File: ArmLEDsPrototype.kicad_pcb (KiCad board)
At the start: 2 copper layers, 11 parts

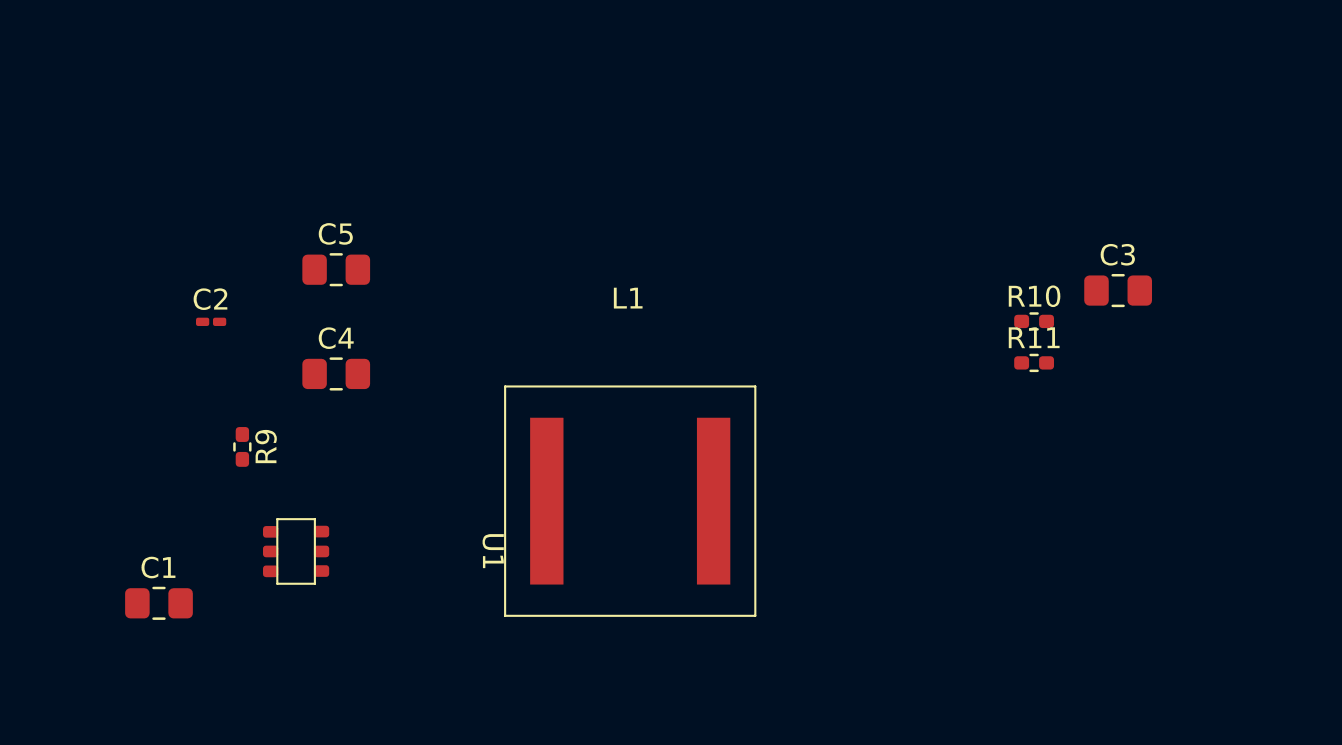
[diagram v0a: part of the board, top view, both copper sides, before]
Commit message: Making PCB
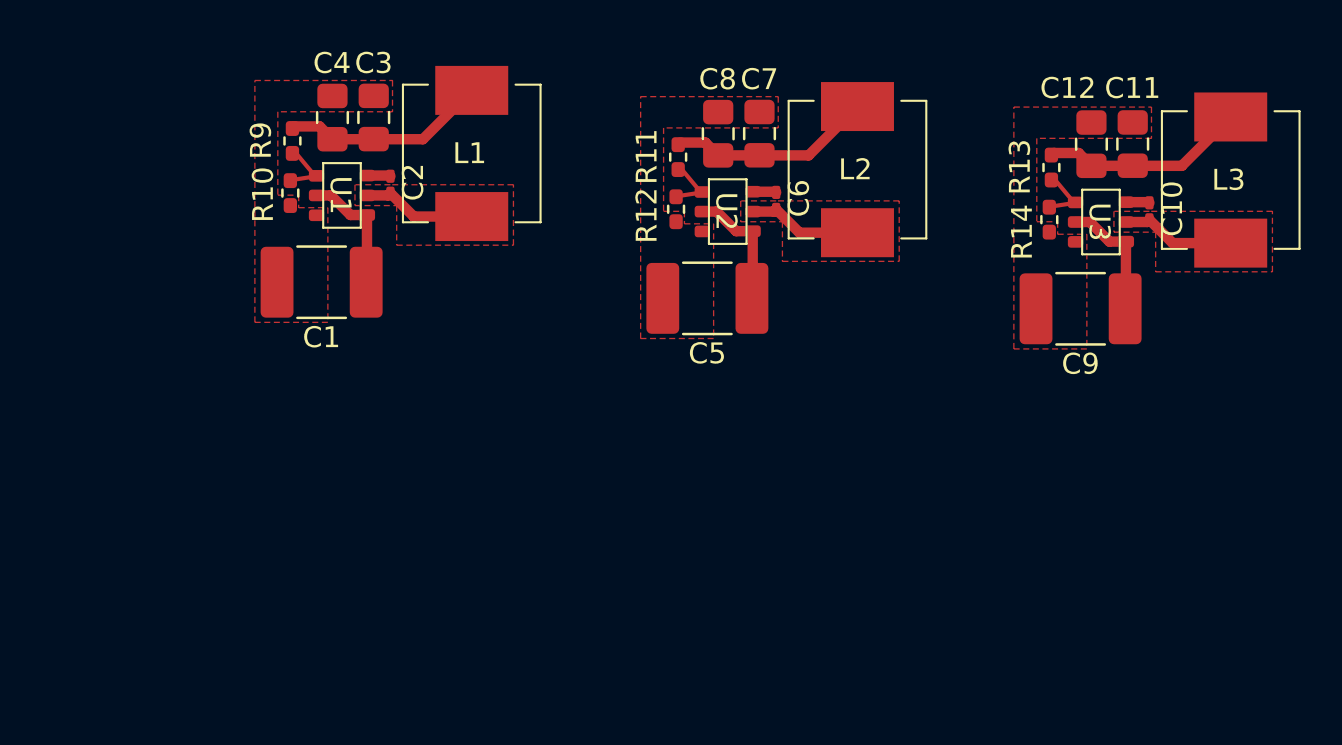
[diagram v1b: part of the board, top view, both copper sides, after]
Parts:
- added C10: C, Capacitor_SMD:C_0201_0603Metric_Pad0.64x0.40mm_HandSolder, F.Cu at (137.5, 25.7)
- added C11: C, Capacitor_SMD:C_0805_2012Metric_Pad1.18x1.45mm_HandSolder, F.Cu at (136.7, 22.5)
- added C12: C, Capacitor_SMD:C_0805_2012Metric_Pad1.18x1.45mm_HandSolder, F.Cu at (134.7, 22.5)
- added C6: C, Capacitor_SMD:C_0201_0603Metric_Pad0.64x0.40mm_HandSolder, F.Cu at (119.6, 25.2)
- added C7: C, Capacitor_SMD:C_0805_2012Metric_Pad1.18x1.45mm_HandSolder, F.Cu at (118.8, 22.0)
- added C8: C, Capacitor_SMD:C_0805_2012Metric_Pad1.18x1.45mm_HandSolder, F.Cu at (116.8, 22.0)
- added C9: C, Capacitor_SMD:C_1812_4532Metric_Pad1.57x3.40mm_HandSolder, F.Cu at (134.2, 30.4)
- added L2: L, ArmLEDFootprintLib:4r7007, F.Cu at (120.2, 23.7)
- added L3: L, ArmLEDFootprintLib:4r7007, F.Cu at (138.1, 24.2)
- added R12: R, Resistor_SMD:R_0402_1005Metric_Pad0.72x0.64mm_HandSolder, F.Cu at (114.8, 25.6)
- added R13: R, Resistor_SMD:R_0402_1005Metric_Pad0.72x0.64mm_HandSolder, F.Cu at (132.8, 23.6)
- added R14: R, Resistor_SMD:R_0402_1005Metric_Pad0.72x0.64mm_HandSolder, F.Cu at (132.7, 26.1)
- added U2: ~, ArmLEDFootprintLib:RT6254A, F.Cu at (117.2, 25.7)
- added U3: ~, ArmLEDFootprintLib:RT6254A, F.Cu at (135.1, 26.2)
- C1, C5: footprint Capacitor_SMD:C_0805_2012Metric_Pad1.18x1.45mm_HandSolder -> Capacitor_SMD:C_1812_4532Metric_Pad1.57x3.40mm_HandSolder
- L1: footprint ArmLEDFootprintLib:Inductor -> ArmLEDFootprintLib:4r7007
- moved C3 36.7 mm to (100.3, 21.2), turned to 90 degrees
- moved R10 36.2 mm to (96.3, 24.8), turned to -90 degrees
- moved R11 19.7 mm to (114.9, 23.1), turned to -90 degrees
- moved C5 17.9 mm to (116.3, 29.9), turned to 180 degrees
- moved C1 17.3 mm to (97.8, 29.1), turned to 180 degrees
- moved U1 17.2 mm to (98.7, 24.9)
- moved R9 14.9 mm to (96.4, 22.3)
- moved C4 12.3 mm to (98.3, 21.2), turned to 90 degrees
- moved L1 12.2 mm to (101.7, 22.9), turned to 90 degrees
- moved C2 10.8 mm to (101.1, 24.4), turned to -90 degrees
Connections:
- A1 pad 30: +5V -> /5V#1
- C3 pad 1: +5V -> /5V#1
- C3 pad 2: Net-(C3-Pad2) -> GND
- C4 pad 1: +5V -> /5V#1
- C5 pad 1: +5V -> +9V
- L1 pad 2: +5V -> /5V#1
- R10 pad 1: +5V -> Net-(U1-FB)
- R10 pad 2: Net-(C3-Pad2) -> GND
- R11 pad 1: GND -> /5V#2
- R11 pad 2: Net-(C3-Pad2) -> Net-(U2-FB)
- R9 pad 1: Net-(U1-FB) -> /5V#1
- R9 pad 2: Net-(C3-Pad2) -> Net-(U1-FB)
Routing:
- net +9V: track 0.00 -> 17.9 mm
- net /5V#2: track 0.00 -> 9.73 mm
- net /5V#1: track 0.00 -> 9.73 mm
- net /5V#3: track 0.00 -> 9.73 mm
- net Net-(U1-LX): track 0.00 -> 5.51 mm
- net Net-(U3-LX): track 0.00 -> 5.51 mm
- net Net-(U2-LX): track 0.00 -> 5.51 mm
- net Net-(U2-BOOT): track 0.00 -> 1.12 mm
- net Net-(U3-BOOT): track 0.00 -> 1.12 mm
- net Net-(U1-BOOT): track 0.00 -> 1.12 mm
- added copper zone on F.Cu, net GND
- added copper zone on F.Cu, net Net-(U1-LX)

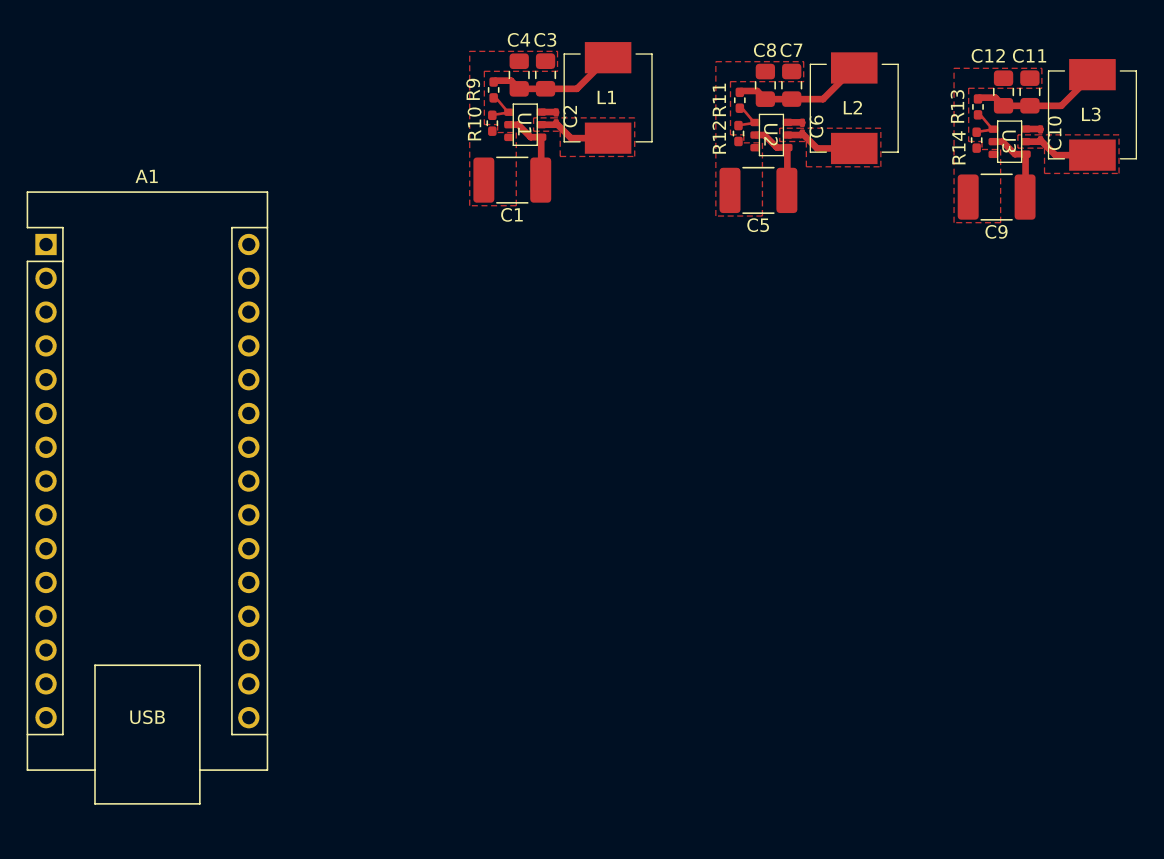
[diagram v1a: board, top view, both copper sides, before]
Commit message: Added parts
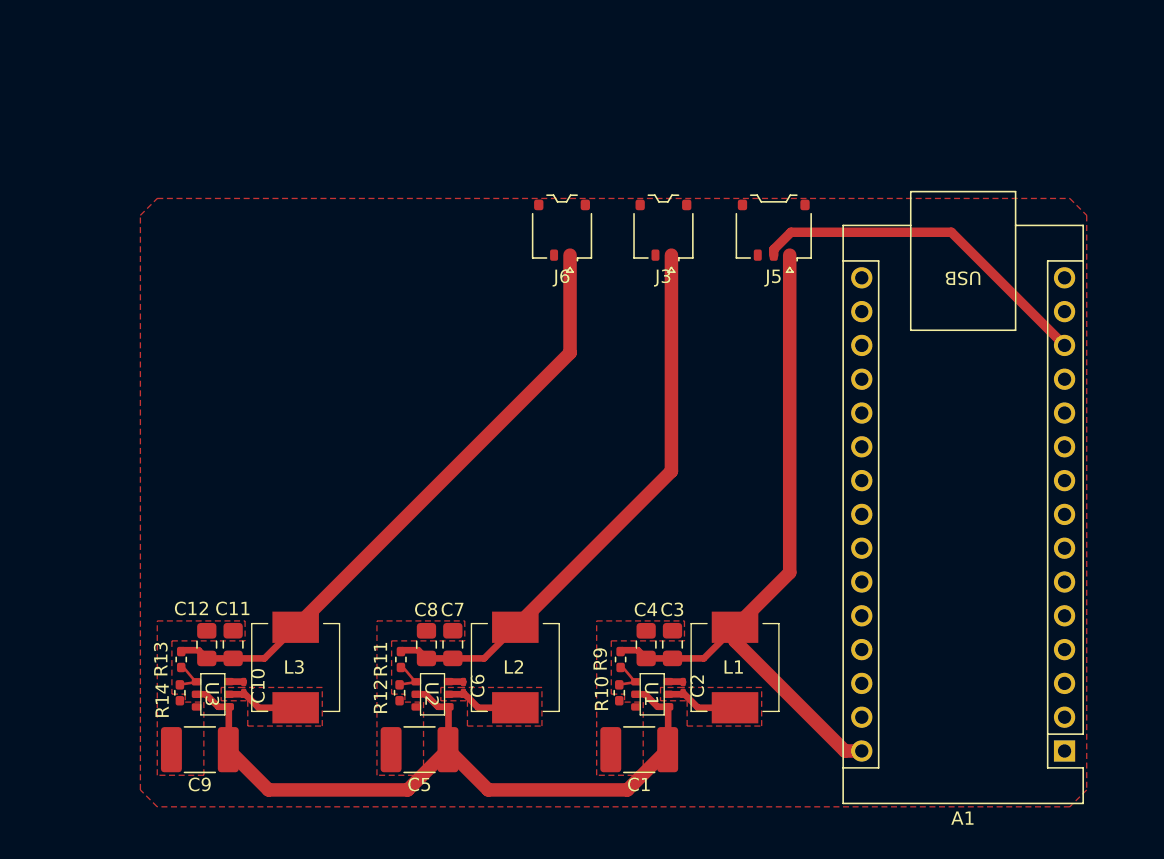
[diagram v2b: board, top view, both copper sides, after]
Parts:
- added J3: Conn_01x02, Connector_Molex:Molex_Pico-EZmate_78171-0002_1x02-1MP_P1.20mm_Vertical, F.Cu at (109.2, 32.9)
- added J5: Conn_01x03, Connector_Molex:Molex_Pico-EZmate_78171-0003_1x03-1MP_P1.20mm_Vertical, F.Cu at (117.5, 32.9)
- added J6: Conn_01x02, Connector_Molex:Molex_Pico-EZmate_78171-0002_1x02-1MP_P1.20mm_Vertical, F.Cu at (101.5, 32.9)
- moved A1 85.5 mm to (139.3, 72.0), turned to 180 degrees
- moved C11 72.9 mm to (76.8, 64.0)
- moved C9 72.9 mm to (74.3, 71.9)
- moved R13 72.9 mm to (72.9, 65.1)
- moved C10 72.9 mm to (77.6, 67.2)
- moved C12 72.9 mm to (74.8, 64.0)
- moved L3 72.9 mm to (78.2, 65.7)
- moved R14 72.9 mm to (72.8, 67.6)
- moved U3 72.9 mm to (75.2, 67.7)
- moved C5 49.1 mm to (90.8, 71.9)
- moved C7 49.1 mm to (93.3, 64.0)
- moved C6 49.1 mm to (94.1, 67.2)
- moved C8 49.1 mm to (91.3, 64.0)
- moved L2 49.1 mm to (94.7, 65.7)
- moved U2 49.1 mm to (91.7, 67.7)
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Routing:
- net /5V#1: track 9.73 -> 53.4 mm
- net +9V: track 17.9 -> 55.9 mm
- net /5V#3: track 9.73 -> 46.2 mm
- net /5V#2: track 9.73 -> 42.5 mm
- net /LED_S: track 0.00 -> 26.3 mm
